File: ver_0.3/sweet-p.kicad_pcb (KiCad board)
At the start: 2 copper layers, 84.3 x 76.2 mm, 51 parts, among them J1 Screw_Terminal_01x02, J2 Conn_01x03_Female, J3 Screw_Terminal_01x03, J4 Conn_01x08_Female, J5 Conn_01x03_Female, J6 Conn_01x06_Female, J7 Screw_Terminal_01x04, J8 Micro_SD_Card, U1 adafruit_tpl511x, U2 MCP1700-3302E_TO, U3 adafruit_ads1115, U4 ssd1306, U5 RFM95W-868S2, U6 Adafruit-Mini-GPS, U7 ds3231

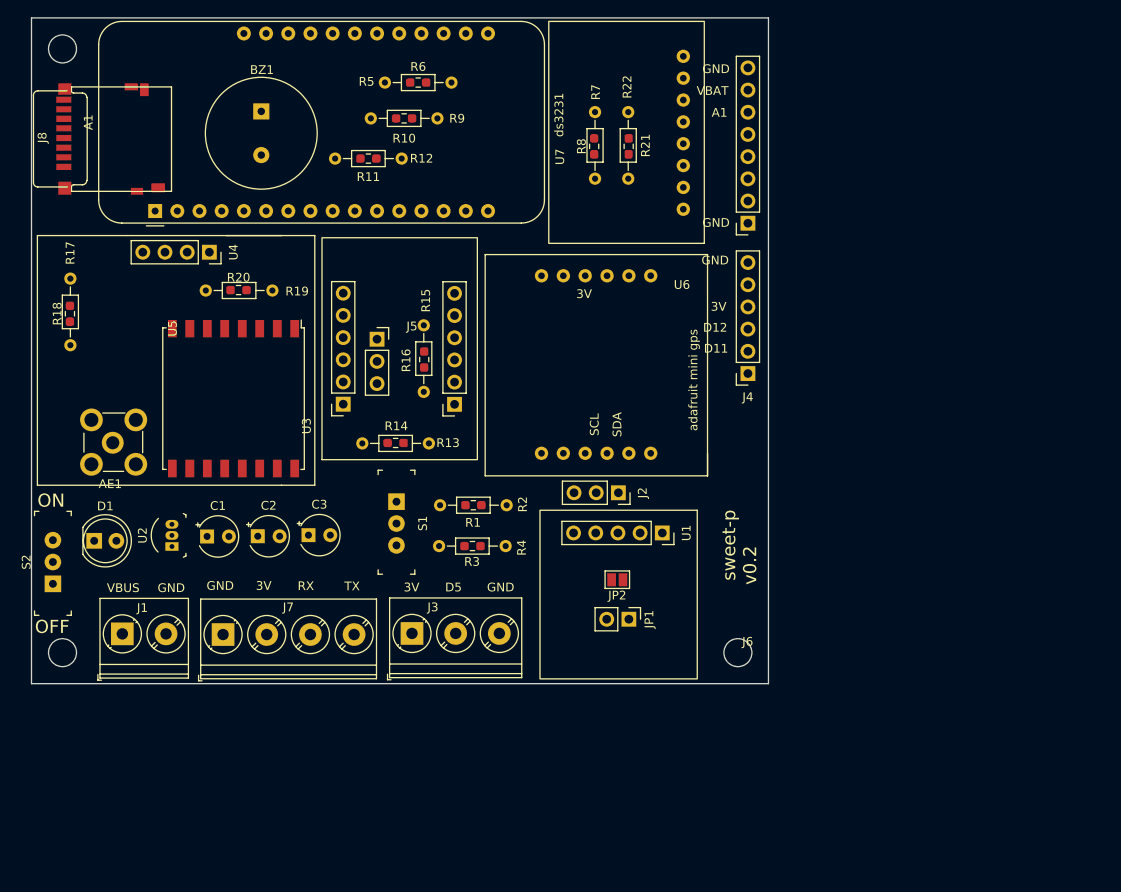
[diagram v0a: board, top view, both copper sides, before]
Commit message: update
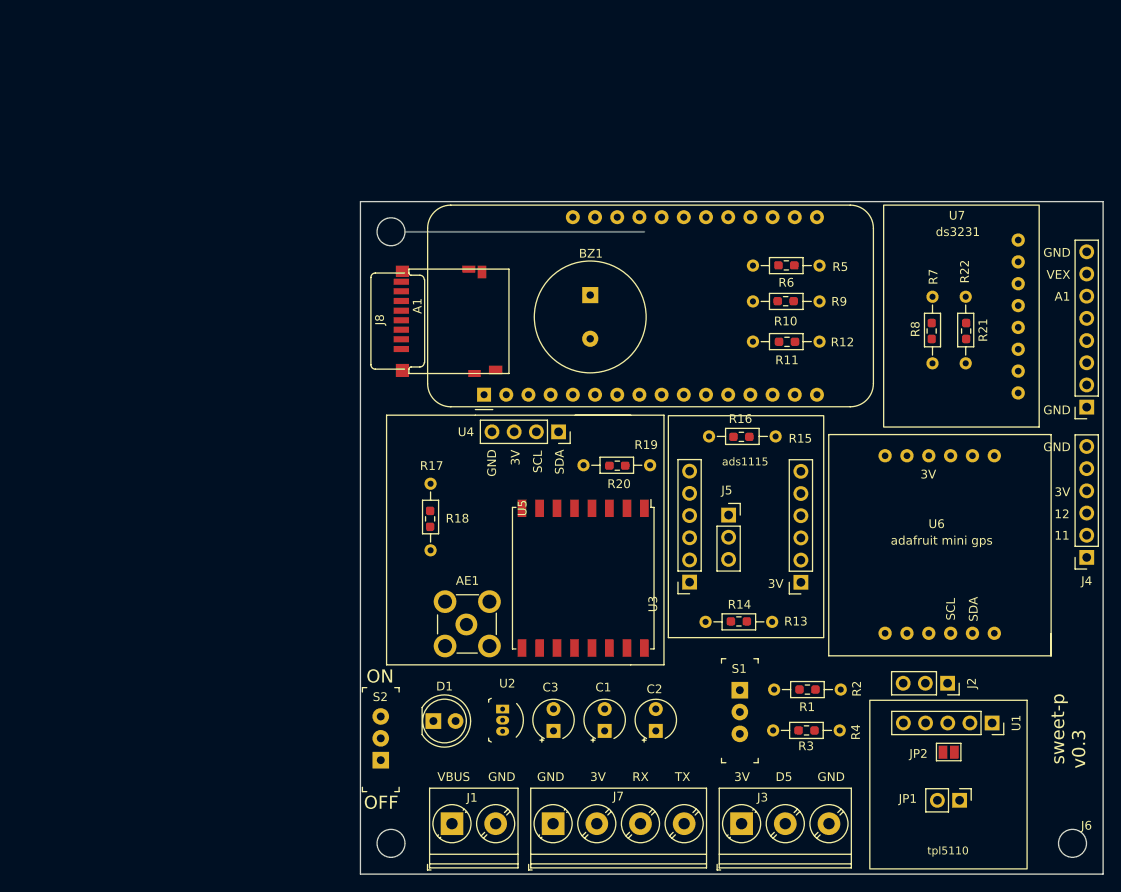
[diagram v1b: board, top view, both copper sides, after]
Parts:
- moved R19 54.6 mm to (58.8, 51.2), turned to 180 degrees
- moved R11 52.3 mm to (74.4, 37.1)
- moved R12 52.2 mm to (70.5, 37.0)
- moved C2 50.7 mm to (59.4, 81.6), turned to 90 degrees
- moved C1 50.7 mm to (53.6, 81.6), turned to 90 degrees
- moved R9 48.5 mm to (78.1, 32.5)
- moved R10 48.4 mm to (74.3, 32.4)
- moved R20 47.8 mm to (55.0, 51.2), turned to 180 degrees
- moved R17 47.4 mm to (33.6, 60.9)
- moved R18 47.4 mm to (33.6, 57.3)
- moved R5 47.0 mm to (70.5, 28.4)
- moved R6 47.0 mm to (74.3, 28.3)
- moved AE1 45.5 mm to (37.8, 69.3)
- moved U5 45.0 mm to (51.1, 64.1)
- moved J5 45.0 mm to (67.7, 56.9)
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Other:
- board size 84.3 x 76.2 mm -> 85 x 77 mm
- board text added: "11"
- board text added: "12"
- board text added: "VEX"
- board text added: "ads1115"
- board text added: "tpl5110"
- board text added: "v0.3"
- board text removed: "D11"
- board text removed: "D12"
- board text removed: "VBAT"
- board text removed: "v0.2"
